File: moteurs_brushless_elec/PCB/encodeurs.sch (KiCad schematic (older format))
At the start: 2 parts, among them U7 Encodeur, U8 Encodeur

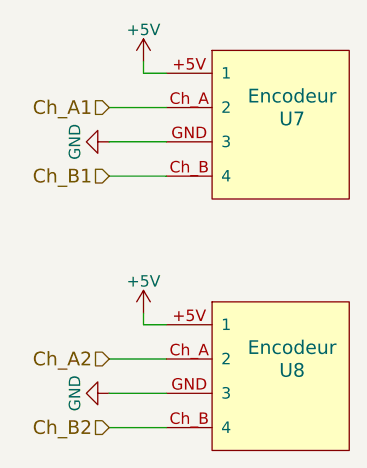
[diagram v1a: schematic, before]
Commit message: routing...
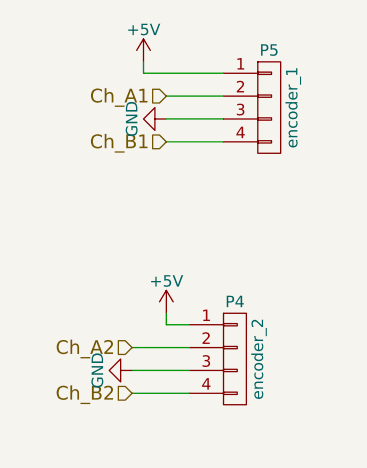
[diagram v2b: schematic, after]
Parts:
- removed U7, U8: Encodeur, Connectors_Molex:Molex_KK-6410-04_04x2.54mm_Straight, symbol Encodeur
- added P4: encoder_2, Connectors_Molex:Molex_KK-6410-04_04x2.54mm_Straight, symbol CONN_01X04
- added P5: encoder_1, Connectors_Molex:Molex_KK-6410-04_04x2.54mm_Straight, symbol CONN_01X04
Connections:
- net +5V: now also P4.1 (P1), P5.1 (P1)
- net Ch_A1: now also P5.2 (P2)
- net Ch_A2: now also P4.2 (P2)
- net Ch_B1: now also P5.4 (P4)
- net Ch_B2: now also P4.4 (P4)
- net GND: now also P4.3 (P3), P5.3 (P3)
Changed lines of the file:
@@
 $EndDescr
-$Comp
-L Encodeur U7
-U 1 1 596AA862
-P 5250 2400
-F 0 "U7" H 5300 2500 60  0000 C CNN
-F 1 "Encodeur" H 5300 2600 60  0000 C CNN
-F 2 "Connectors_Molex:Molex_KK-6410-04_04x2.54mm_Straight" H 5250 2400 60  0001 C CNN
-F 3 "" H 5250 2400 60  0001 C CNN
-	1    5250 2400
-	1    0    0    -1
-$EndComp
-$Comp
-L Encodeur U8
-U 1 1 596AA88D
-P 5250 3500
-F 0 "U8" H 5300 3600 60  0000 C CNN
-F 1 "Encodeur" H 5300 3700 60  0000 C CNN
-F 2 "Connectors_Molex:Molex_KK-6410-04_04x2.54mm_Straight" H 5250 3500 60  0001 C CNN
-F 3 "" H 5250 3500 60  0001 C CNN
-	1    5250 3500
-	1    0    0    -1
-$EndComp
 $Comp
 L +5V #PWR060
@@
 L +5V #PWR061
 U 1 1 596AAFB0
-P 4650 3150
-F 0 "#PWR061" H 4650 3000 50  0001 C CNN
-F 1 "+5V" H 4650 3290 50  0000 C CNN
-F 2 "" H 4650 3150 50  0001 C CNN
-F 3 "" H 4650 3150 50  0001 C CNN
-	1    4650 3150
+P 4750 3150
+F 0 "#PWR061" H 4750 3000 50  0001 C CNN
+F 1 "+5V" H 4750 3290 50  0000 C CNN
+F 2 "" H 4750 3150 50  0001 C CNN
+F 3 "" H 4750 3150 50  0001 C CNN
+	1    4750 3150
 	1    0    0    -1
 $EndComp
@@
 L GND #PWR062
 U 1 1 596AB08B
-P 4500 2400
-F 0 "#PWR062" H 4500 2150 50  0001 C CNN
-F 1 "GND" H 4500 2250 50  0000 C CNN
-F 2 "" H 4500 2400 50  0001 C CNN
-F 3 "" H 4500 2400 50  0001 C CNN
-	1    4500 2400
+P 4750 2300
+F 0 "#PWR062" H 4750 2050 50  0001 C CNN
+F 1 "GND" H 4750 2150 50  0000 C CNN
+F 2 "" H 4750 2300 50  0001 C CNN
+F 3 "" H 4750 2300 50  0001 C CNN
+	1    4750 2300
 	0    1    1    0
 $EndComp
@@
 L GND #PWR063
 U 1 1 596AB0FD
-P 4500 3500
-F 0 "#PWR063" H 4500 3250 50  0001 C CNN
-F 1 "GND" H 4500 3350 50  0000 C CNN
-F 2 "" H 4500 3500 50  0001 C CNN
-F 3 "" H 4500 3500 50  0001 C CNN
-	1    4500 3500
+P 4600 3400
+F 0 "#PWR063" H 4600 3150 50  0001 C CNN
+F 1 "GND" H 4600 3250 50  0000 C CNN
+F 2 "" H 4600 3400 50  0001 C CNN
+F 3 "" H 4600 3400 50  0001 C CNN
+	1    4600 3400
 	0    1    1    0
 $EndComp
-Text HLabel 4500 2250 0    60   Input ~ 0
+Text HLabel 4750 2200 0    60   Input ~ 0
 Ch_A1
-Text HLabel 4500 2550 0    60   Input ~ 0
+Text HLabel 4750 2400 0    60   Input ~ 0
 Ch_B1
-Text HLabel 4500 3350 0    60   Input ~ 0
+Text HLabel 4600 3300 0    60   Input ~ 0
 Ch_A2
-Text HLabel 4500 3650 0    60   Input ~ 0
+Text HLabel 4600 3500 0    60   Input ~ 0
 Ch_B2
 Wire Wire Line
 	4650 2050 4650 2100
 Wire Wire Line
-	4650 2100 4750 2100
+	4650 2100 5000 2100
 Wire Wire Line
-	4500 2250 4750 2250
+	4750 2200 5000 2200
 Wire Wire Line
-	4500 2400 4750 2400
+	4750 2300 5000 2300
 Wire Wire Line
-	4500 2550 4750 2550
+	4750 2400 5000 2400
 Wire Wire Line
-	4650 3150 4650 3200
+	4750 3150 4750 3200
 Wire Wire Line
-	4650 3200 4750 3200
+	4750 3200 4850 3200
 Wire Wire Line
-	4500 3350 4750 3350
+	4600 3300 4850 3300
 Wire Wire Line
-	4500 3500 4750 3500
+	4600 3400 4850 3400
 Wire Wire Line
-	4500 3650 4750 3650
+	4600 3500 4850 3500
+$Comp
+L CONN_01X04 P5
+U 1 1 59C30399
+P 5200 2250
+F 0 "P5" H 5200 2500 50  0000 C CNN
+F 1 "encoder_1" V 5300 2250 50  0000 C CNN
+F 2 "Connectors_Molex:Molex_KK-6410-04_04x2.54mm_Straight" H 5200 2250 50  0001 C CNN
+F 3 "" H 5200 2250 50  0000 C CNN
+	1    5200 2250
+	1    0    0    -1
+$EndComp
+$Comp
+L CONN_01X04 P4
+U 1 1 59C303CC
+P 5050 3350
+F 0 "P4" H 5050 3600 50  0000 C CNN
+F 1 "encoder_2" V 5150 3350 50  0000 C CNN
+F 2 "Connectors_Molex:Molex_KK-6410-04_04x2.54mm_Straight" H 5050 3350 50  0001 C CNN
+F 3 "" H 5050 3350 50  0000 C CNN
+	1    5050 3350
+	1    0    0    -1
+$EndComp
 $EndSCHEMATC
